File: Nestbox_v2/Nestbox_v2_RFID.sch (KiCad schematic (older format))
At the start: 6 parts

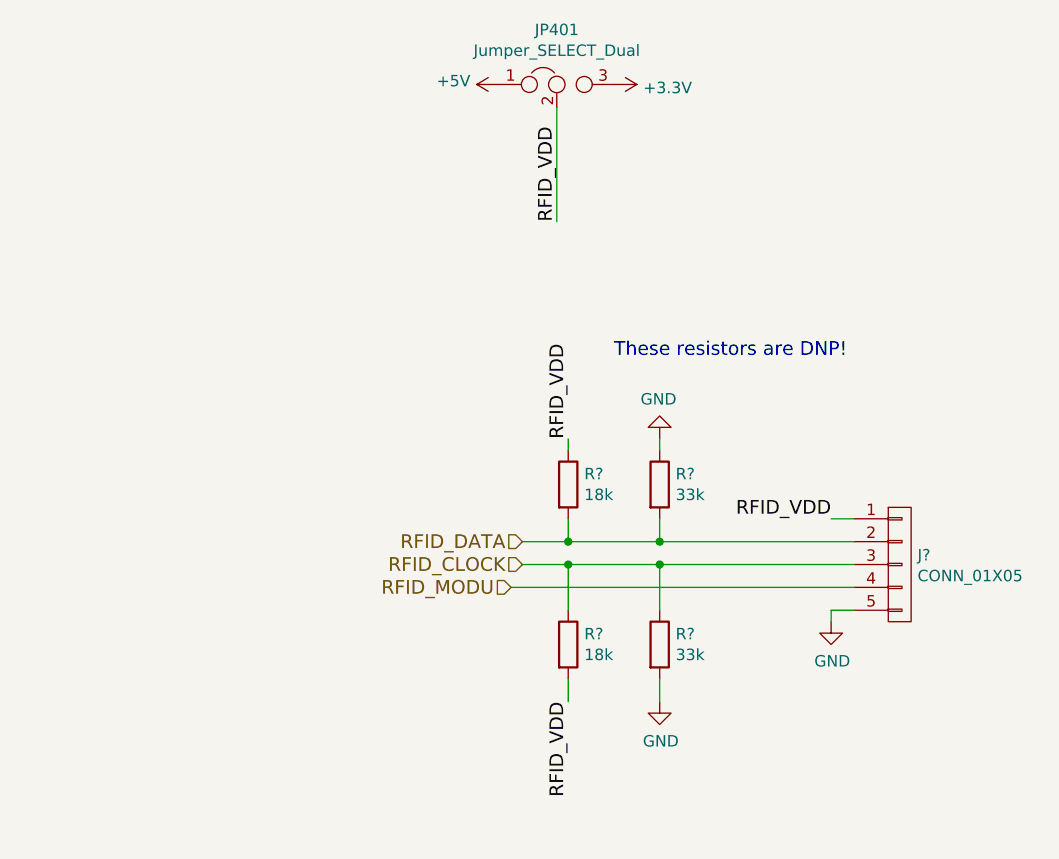
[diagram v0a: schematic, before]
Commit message: finished power supply schematics
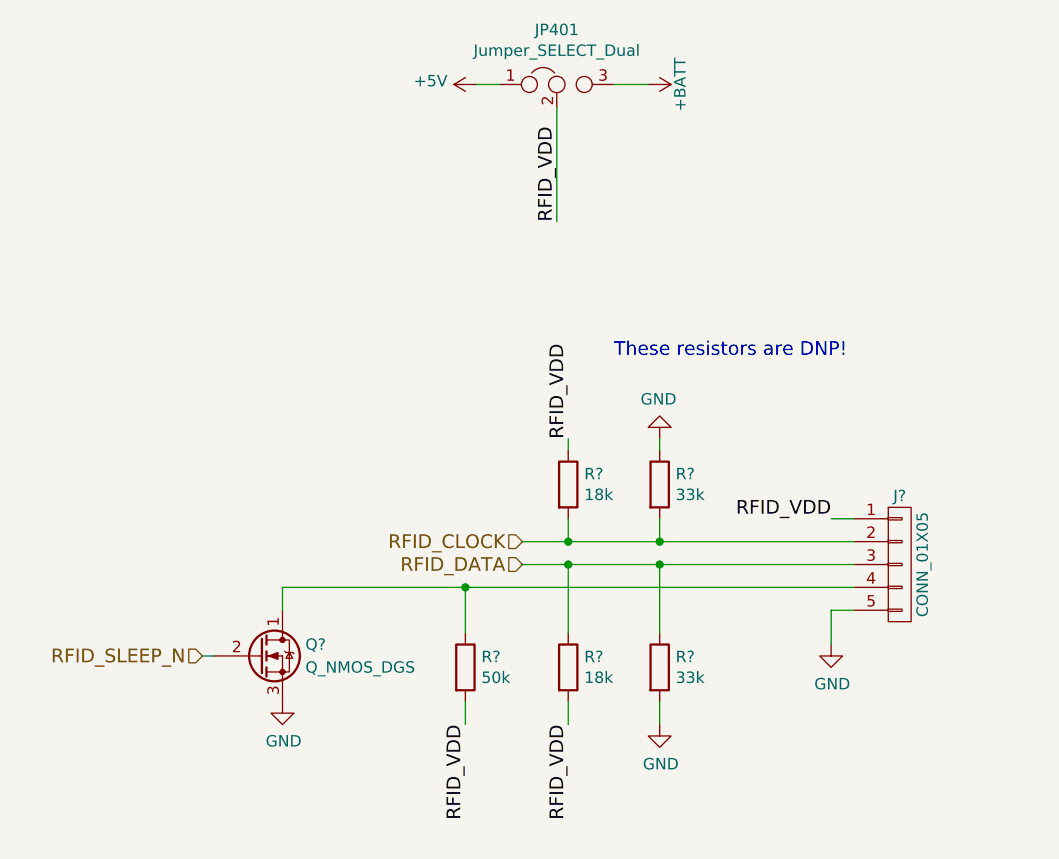
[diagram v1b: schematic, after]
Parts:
- removed J?: CONN_01X05, symbol CONN_01X05
- added J?: CONN_01X05, symbol CONN_01X05
- added Q?: Q_NMOS_DGS, symbol Q_NMOS_DGS
- added R?: 50k, symbol R
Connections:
- net GND: now also J?.5 (P5), Q?.3 (S)
- net RFID_CLOCK: now also R?.2, R?.2, J?.2 (P2); no longer R?.1, R?.1
- net RFID_DATA: now also R?.1, R?.1, J?.3 (P3); no longer R?.2, R?.2
- net RFID_VDD: now also J?.1 (P1), R?.2
- net +3V3 renamed +BATT
- new net: J?.4 (P4), Q?.1 (D), R?.1
- new net RFID_SLEEP_N: Q?.2 (G)
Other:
- moved on the sheet: R?
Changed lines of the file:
@@
 Comment4 ""
 $EndDescr
-$Comp
-L +3.3V #PWR048
-U 1 1 59FF36B1
-P 5800 2300
-F 0 "#PWR048" H 5800 2150 50  0001 C CNN
-F 1 "+3.3V" V 5815 2428 50  0000 L CNN
-F 2 "" H 5800 2300 50  0000 C CNN
-F 3 "" H 5800 2300 50  0000 C CNN
-	1    5800 2300
-	0    1    1    0
-$EndComp
 Text Label 6750 4200 2    60   ~ 0
 RFID_VDD
@@
 L +5V #PWR049
 U 1 1 5A0305A8
-P 5300 2300
-F 0 "#PWR049" H 5300 2150 50  0001 C CNN
-F 1 "+5V" V 5315 2428 50  0000 L CNN
-F 2 "" H 5300 2300 50  0001 C CNN
-F 3 "" H 5300 2300 50  0001 C CNN
-	1    5300 2300
+P 5200 2300
+F 0 "#PWR049" H 5200 2150 50  0001 C CNN
+F 1 "+5V" V 5215 2428 50  0000 L CNN
+F 2 "" H 5200 2300 50  0001 C CNN
+F 3 "" H 5200 2300 50  0001 C CNN
+	1    5200 2300
 	0    -1   -1   0
 $EndComp
@@
 L R R?
 U 1 1 5AF8A741
-P 5600 4750
-F 0 "R?" H 5670 4796 50  0000 L CNN
-F 1 "18k" H 5670 4705 50  0000 L CNN
-F 2 "" V 5530 4750 50  0001 C CNN
-F 3 "" H 5600 4750 50  0001 C CNN
-	1    5600 4750
+P 5600 4850
+F 0 "R?" H 5670 4896 50  0000 L CNN
+F 1 "18k" H 5670 4805 50  0000 L CNN
+F 2 "" V 5530 4850 50  0001 C CNN
+F 3 "" H 5600 4850 50  0001 C CNN
+	1    5600 4850
 	1    0    0    -1
 $EndComp
@@
 L R R?
 U 1 1 5AF8AB4E
-P 6000 4750
-F 0 "R?" H 6070 4796 50  0000 L CNN
-F 1 "33k" H 6070 4705 50  0000 L CNN
-F 2 "" V 5930 4750 50  0001 C CNN
-F 3 "" H 6000 4750 50  0001 C CNN
-	1    6000 4750
+P 6000 4850
+F 0 "R?" H 6070 4896 50  0000 L CNN
+F 1 "33k" H 6070 4805 50  0000 L CNN
+F 2 "" V 5930 4850 50  0001 C CNN
+F 3 "" H 6000 4850 50  0001 C CNN
+	1    6000 4850
 	1    0    0    -1
 $EndComp
@@
 L GND #PWR?
 U 1 1 5AF8AC8E
-P 6000 5000
-F 0 "#PWR?" H 6000 4750 50  0001 C CNN
-F 1 "GND" H 6005 4827 50  0000 C CNN
-F 2 "" H 6000 5000 50  0001 C CNN
-F 3 "" H 6000 5000 50  0001 C CNN
-	1    6000 5000
-	1    0    0    -1
-$EndComp
-Wire Wire Line
-	6000 4900 6000 5000
+P 6000 5100
+F 0 "#PWR?" H 6000 4850 50  0001 C CNN
+F 1 "GND" H 6005 4927 50  0000 C CNN
+F 2 "" H 6000 5100 50  0001 C CNN
+F 3 "" H 6000 5100 50  0001 C CNN
+	1    6000 5100
+	1    0    0    -1
+$EndComp
+Wire Wire Line
+	6000 5000 6000 5100
 Wire Wire Line
 	6000 3900 6000 3850
 Connection ~ 6000 4400
 Wire Wire Line
-	6000 4400 6000 4600
+	6000 4400 6000 4700
 Connection ~ 6000 4300
 Wire Wire Line
 	6000 4300 6000 4200
 Wire Wire Line
-	5600 4900 5600 5000
+	5600 5000 5600 5100
 Wire Wire Line
 	5600 3850 5600 3900
@@
 Connection ~ 5600 4400
 Wire Wire Line
-	5600 4400 5600 4600
-Wire Wire Line
-	5350 4500 6850 4500
+	5600 4400 5600 4700
 Wire Wire Line
 	5400 4400 6850 4400
@@
 Text Label 5600 3850 1    60   ~ 0
 RFID_VDD
-Text Label 5600 5000 3    60   ~ 0
-RFID_VDD
+Text Label 5600 5100 3    60   ~ 0
+RFID_VDD
+$Comp
+L GND #PWR?
+U 1 1 5AF8B903
+P 6750 4750
+F 0 "#PWR?" H 6750 4500 50  0001 C CNN
+F 1 "GND" H 6755 4577 50  0000 C CNN
+F 2 "" H 6750 4750 50  0001 C CNN
+F 3 "" H 6750 4750 50  0001 C CNN
+	1    6750 4750
+	1    0    0    -1
+$EndComp
+Text HLabel 5400 4400 0    60   Input ~ 0
+RFID_DATA
+Text HLabel 5400 4300 0    60   Input ~ 0
+RFID_CLOCK
+Text Notes 5800 3500 0    60   ~ 0
+These resistors are DNP!\n
+$Comp
+L Q_NMOS_DGS Q?
+U 1 1 5B08713B
+P 4250 4800
+F 0 "Q?" H 4450 4850 50  0000 L CNN
+F 1 "Q_NMOS_DGS" H 4450 4750 50  0000 L CNN
+F 2 "" H 4450 4900 50  0001 C CNN
+F 3 "" H 4250 4800 50  0001 C CNN
+	1    4250 4800
+	1    0    0    -1
+$EndComp
+Text Label 5150 5100 3    60   ~ 0
+RFID_VDD
+Wire Wire Line
+	5150 5100 5150 5000
+$Comp
+L GND #PWR?
+U 1 1 5B088780
+P 4350 5000
+F 0 "#PWR?" H 4350 4750 50  0001 C CNN
+F 1 "GND" H 4355 4827 50  0000 C CNN
+F 2 "" H 4350 5000 50  0001 C CNN
+F 3 "" H 4350 5000 50  0001 C CNN
+	1    4350 5000
+	1    0    0    -1
+$EndComp
+Text HLabel 4000 4800 0    60   Input ~ 0
+RFID_SLEEP_N
+Wire Wire Line
+	4000 4800 4050 4800
+Wire Wire Line
+	4350 4600 4350 4500
+Wire Wire Line
+	4350 4500 6850 4500
+$Comp
+L R R?
+U 1 1 5B088617
+P 5150 4850
+F 0 "R?" H 5220 4896 50  0000 L CNN
+F 1 "50k" H 5220 4805 50  0000 L CNN
+F 2 "" V 5080 4850 50  0001 C CNN
+F 3 "" H 5150 4850 50  0001 C CNN
+	1    5150 4850
+	1    0    0    -1
+$EndComp
+Wire Wire Line
+	5150 4700 5150 4500
+Connection ~ 5150 4500
+Wire Wire Line
+	6750 4600 6850 4600
 $Comp
 L CONN_01X05 J?
-U 1 1 5AF8B87E
+U 1 1 5B08A8CB
 P 7050 4400
-F 0 "J?" H 7128 4441 50  0000 L CNN
-F 1 "CONN_01X05" H 7128 4350 50  0000 L CNN
+F 0 "J?" H 7050 4700 50  0000 C CNN
+F 1 "CONN_01X05" V 7150 4400 50  0000 C CNN
 F 2 "" H 7050 4400 50  0001 C CNN
 F 3 "" H 7050 4400 50  0001 C CNN
@@
 	1    0    0    -1
 $EndComp
-$Comp
-L GND #PWR?
-U 1 1 5AF8B903
-P 6750 4650
-F 0 "#PWR?" H 6750 4400 50  0001 C CNN
-F 1 "GND" H 6755 4477 50  0000 C CNN
-F 2 "" H 6750 4650 50  0001 C CNN
-F 3 "" H 6750 4650 50  0001 C CNN
-	1    6750 4650
-	1    0    0    -1
-$EndComp
-Wire Wire Line
-	6850 4600 6750 4600
-Wire Wire Line
-	6750 4600 6750 4650
-Text HLabel 5400 4300 0    60   Input ~ 0
-RFID_DATA
-Text HLabel 5400 4400 0    60   Input ~ 0
-RFID_CLOCK
-Text HLabel 5350 4500 0    60   Input ~ 0
-RFID_MODU
-Text Notes 5800 3500 0    60   ~ 0
-These resistors are DNP!\n
+Wire Wire Line
+	6750 4750 6750 4600
+Wire Wire Line
+	5800 2300 5950 2300
+Wire Wire Line
+	5200 2300 5300 2300
+$Comp
+L +BATT #PWR?
+U 1 1 5B08AE2C
+P 5950 2300
+F 0 "#PWR?" H 5950 2150 50  0001 C CNN
+F 1 "+BATT" H 5950 2440 50  0000 C CNN
+F 2 "" H 5950 2300 50  0001 C CNN
+F 3 "" H 5950 2300 50  0001 C CNN
+	1    5950 2300
+	0    1    1    0
+$EndComp
 $EndSCHEMATC
